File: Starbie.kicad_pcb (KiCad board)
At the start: 2 copper layers, 7 parts, among them SW1 SW_Push, SW2 SW_Push, U1 XIAO-ESP32-C3-SMD, U4 DHT11

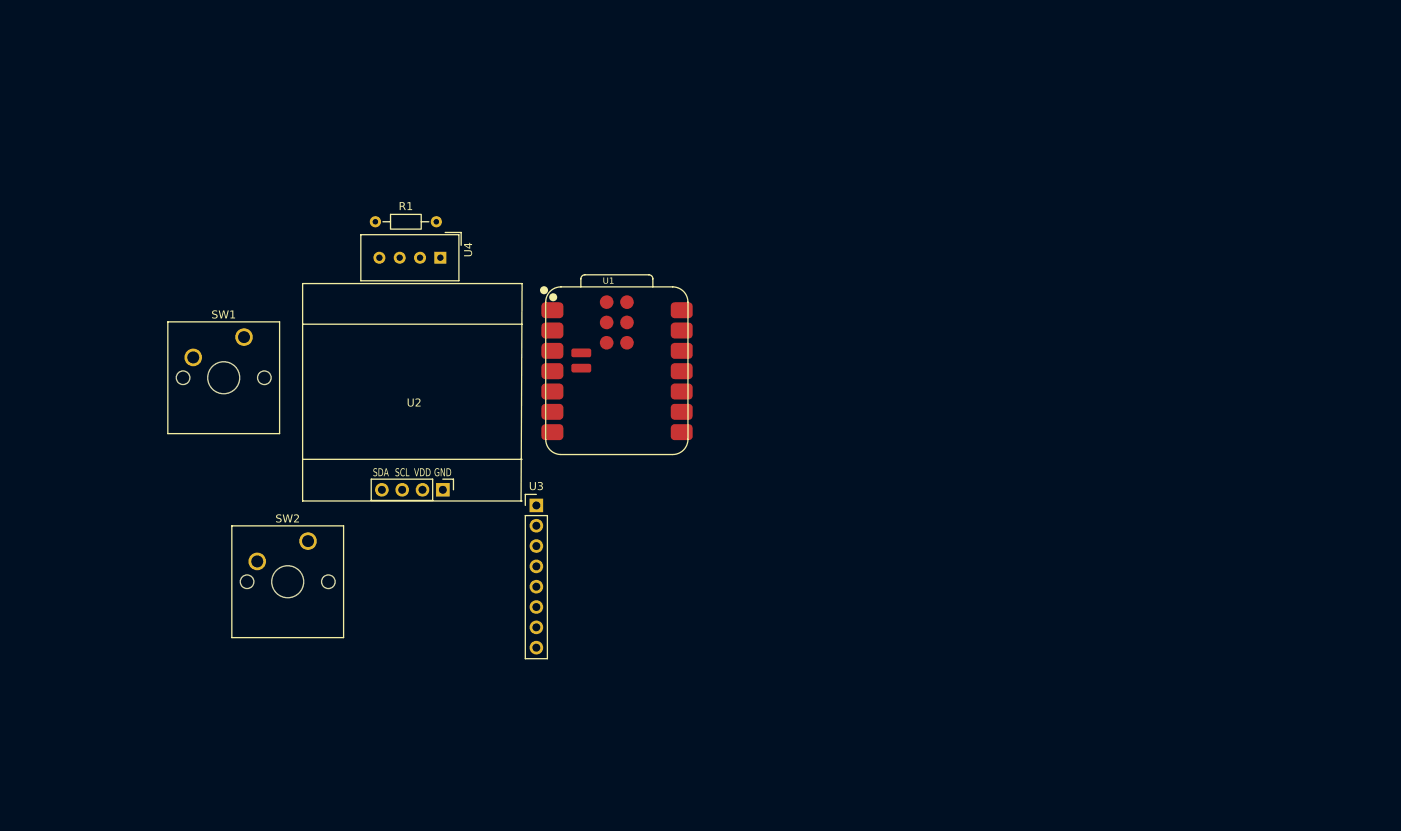
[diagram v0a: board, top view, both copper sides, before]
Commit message: Finished the PCB, and exported.
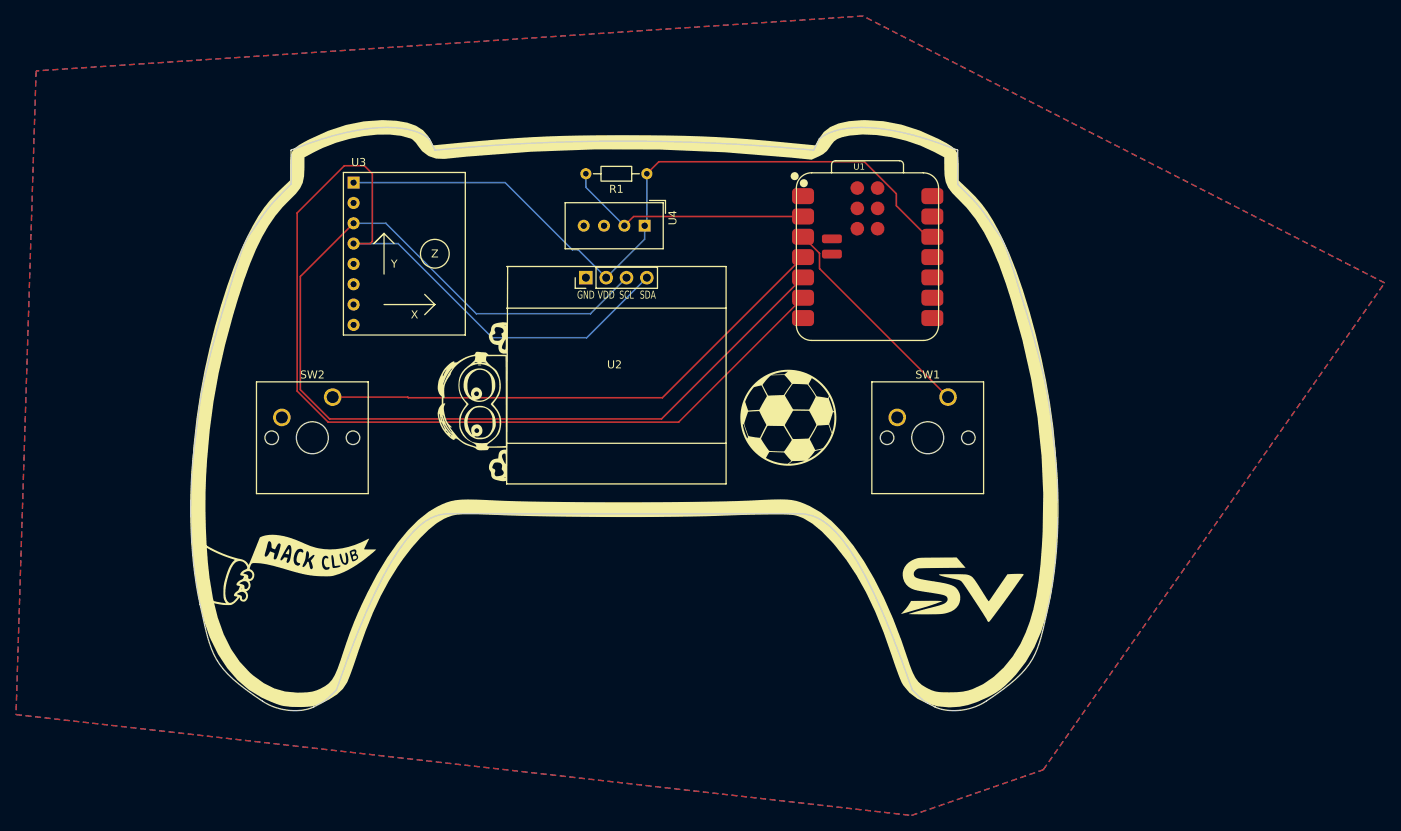
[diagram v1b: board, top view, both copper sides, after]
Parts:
- added G***: LOGO, LOGO, F.Cu at (227.0, 91.5)
- added G***: LOGO, LOGO, F.Cu at (143.0, 89.5)
- added G***: LOGO, LOGO, F.Cu at (185.0, 70.0)
- added G***: LOGO, LOGO, F.Cu at (205.5, 70.5)
- added G***: LOGO, LOGO, F.Cu at (164.7, 68.5)
- added G***: LOGO, LOGO, B.Cu at (160.5, 75.0)
- U3: footprint Connector_PinHeader_2.54mm:PinHeader_1x08_P2.54mm_Vertical -> Imported Parts:MPU6050_Module
- moved SW1 88.3 mm to (225.5, 67.9)
- moved U3 46.4 mm to (151.2, 41.1)
- moved U2 36.8 mm to (184.0, 53.0), turned to 0 degrees
- moved R1 34.5 mm to (187.8, 40.0), turned to 180 degrees
- moved U1 34.4 mm to (206.5, 60.9)
- moved U4 25.9 mm to (187.5, 46.5)
- moved SW2 18.3 mm to (148.5, 67.9)
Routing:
- net /SDA: track 0.00 -> 161.4 mm
- net /SCL: track 0.00 -> 135.9 mm
- net +3.3V: track 0.00 -> 92.7 mm
- net /GPIO3: track 0.00 -> 66.1 mm
- net /DHT11 DATA: track 0.00 -> 31.3 mm
- net /GPIO2: track 0.00 -> 27.5 mm
- added copper zone on B.Cu, net GND
- added copper zone on F.Cu, net GND
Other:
- board outline added: 108.4 x 72.9 mm
